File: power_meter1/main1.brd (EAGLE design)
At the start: 86 x 42 mm, 41 parts, among them IC1 7805TV, Q1 16M, U1 LT1999CS8-50PBF, U2 ATMEGA168PA-AU, X1 SCREWTERM_5MM_4WAY

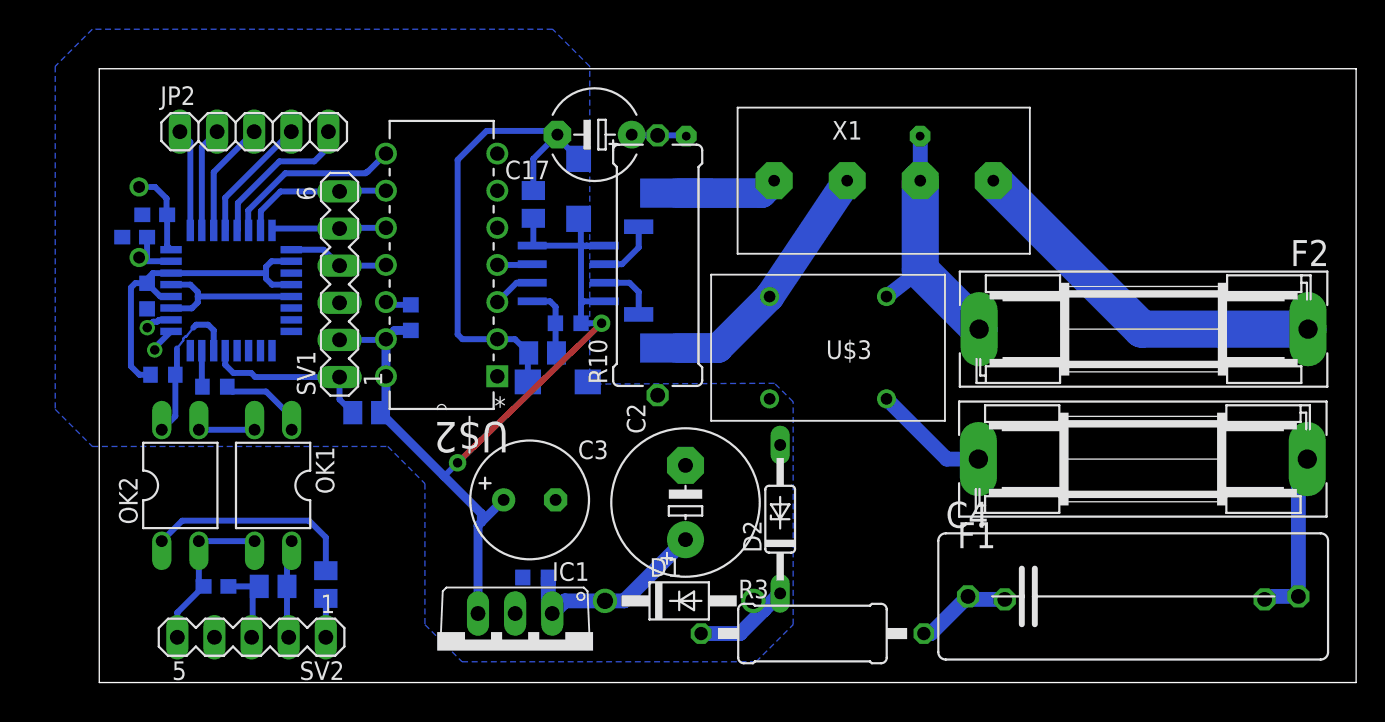
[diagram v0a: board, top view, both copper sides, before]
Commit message: a
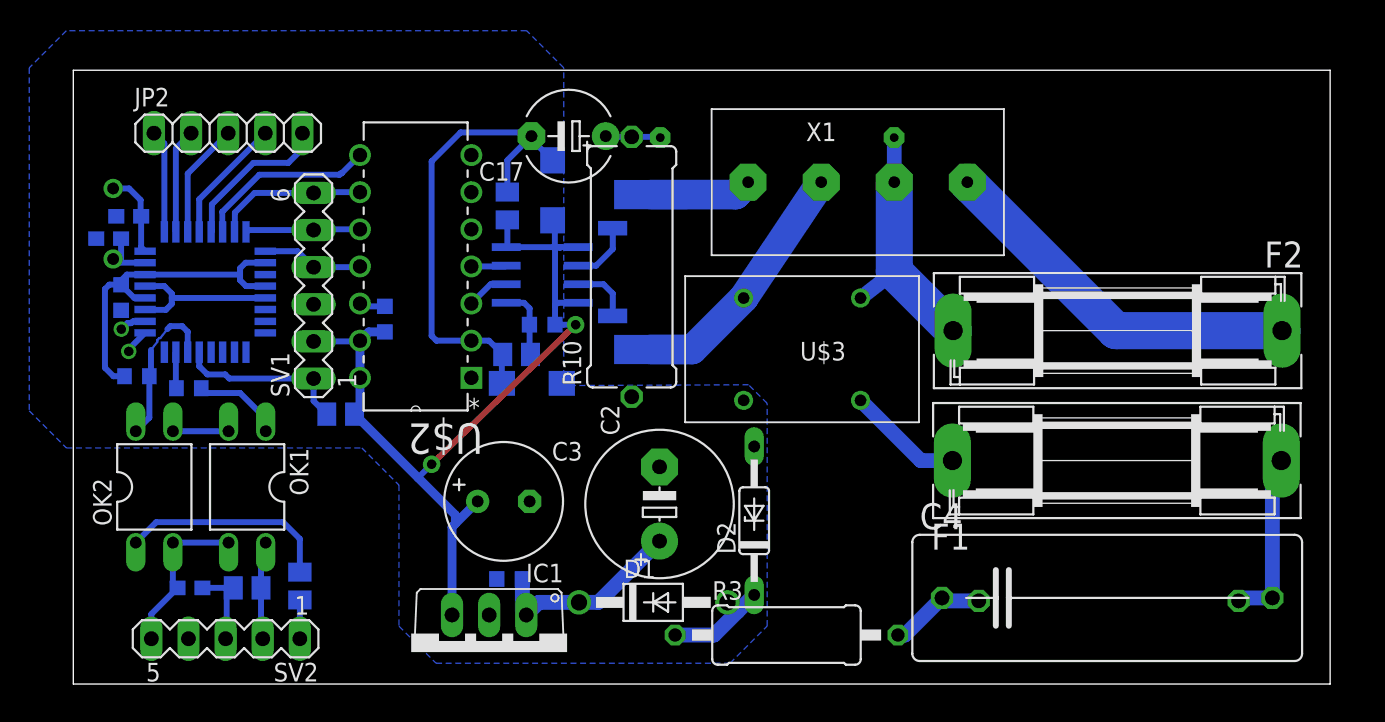
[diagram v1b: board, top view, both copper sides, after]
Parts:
- moved D2 1.78 mm to (46.8, 11.1)
- moved F1 1.78 mm to (71.6, 15.2)
- moved F2 1.78 mm to (71.7, 24.1)
- moved R4 1.78 mm to (71.1, 5.59)
- moved C9 1.78 mm to (30.1, 7.09)
- moved R12 1.78 mm to (29.9, 32.6)
- moved R11 1.78 mm to (30.6, 22.5)
- moved U$2 1.78 mm to (19.8, 36.1)
- moved C8 1.78 mm to (8.20, 6.48)
- moved JP2 1.78 mm to (10.8, 37.6)
- moved OK1 1.78 mm to (12.1, 13.4)
- moved OK2 1.78 mm to (5.77, 13.4)
- moved R1 1.78 mm to (12.1, 6.48)
- moved R7 1.78 mm to (8.13, 20.1)
- moved SV2 1.78 mm to (10.6, 3.00)
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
